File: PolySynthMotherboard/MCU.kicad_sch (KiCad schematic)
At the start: 45 parts, among them J201 SWD Header, J202 USB_C_Receptacle_USB2.0, J203 MIDI_In, J204 MIDI_Thru, J205 MIDI_Out, J401 Micro_SD_Card_Det2, SW201 RST, SW202 BOOT, U201 STM32F411RETx, U202 74HC595, U203 74HC595, U204 4N35, U205 74HC04, Y201 16MHz, Y202 32.768kHZ

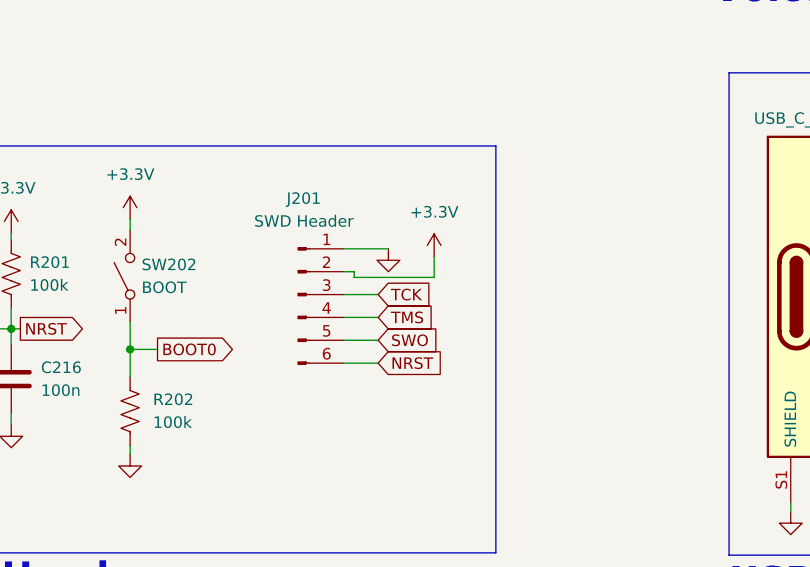
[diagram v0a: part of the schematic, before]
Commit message: board layout
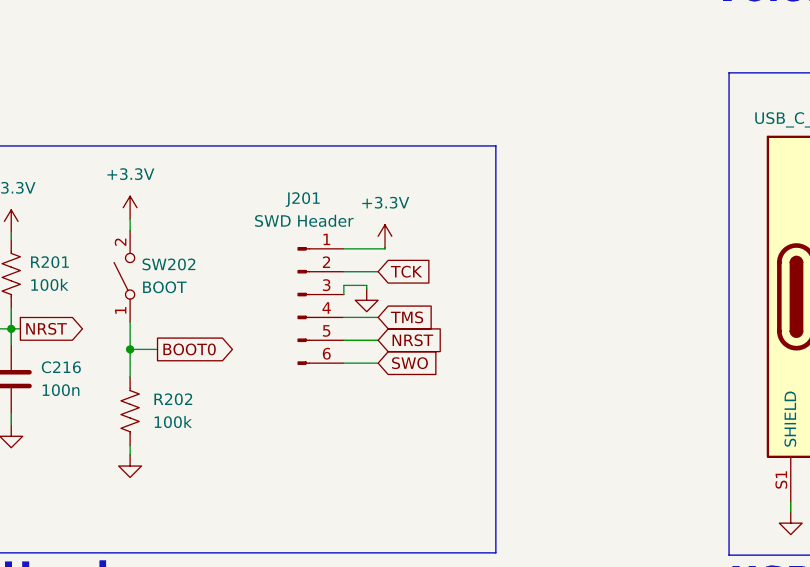
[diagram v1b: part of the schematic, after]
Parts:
- D201: footprint Diode_THT:D_DO-35_SOD27_P7.62mm_Horizontal -> Diode_SMD:D_SOD-123
- U205: footprint PCM_Package_SO_AKL:SOIC-14_3.9x8.7mm_P1.27mm -> Package_SO:SOIC-14_3.9x8.7mm_P1.27mm
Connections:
- net +3.3V: now also J201.1 (Pin_1); no longer J201.2 (Pin_2)
- net GND: now also J201.3 (Pin_3); no longer J201.1 (Pin_1)
- net NRST: now also J201.5 (Pin_5); no longer J201.6 (Pin_6)
- net SWO: now also J201.6 (Pin_6); no longer J201.5 (Pin_5)
- net TCK: now also J201.2 (Pin_2); no longer J201.3 (Pin_3)
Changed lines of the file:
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@@
     (stroke (width 0) (type default))
   )
+  (wire (pts (xy 115.951 196.342) (xy 115.951 196.723))
+    (stroke (width 0) (type default))
+  )
   (wire (pts (xy 121.158 93.218) (xy 123.698 93.218))
     (stroke (width 0) (type default))
@@
     (stroke (width 0) (type default))
   )
-  (wire (pts (xy 114.554 194.818) (xy 114.554 195.453))
-    (stroke (width 0) (type default))
-  )
   (wire (pts (xy 34.29 109.474) (xy 34.29 121.92))
     (stroke (width 0) (type default))
@@
     (stroke (width 0) (type default))
   )
-  (wire (pts (xy 113.411 197.358) (xy 117.221 197.358))
+  (wire (pts (xy 113.411 194.818) (xy 117.221 194.818))
     (stroke (width 0) (type default))
   )
@@
     (stroke (width 0) (type default))
   )
-  (wire (pts (xy 114.554 195.453) (xy 123.444 195.453))
-    (stroke (width 0) (type default))
-  )
   (wire (pts (xy 81.026 85.598) (xy 85.598 85.598))
     (stroke (width 0) (type default))
@@
     (stroke (width 0) (type default))
   )
+  (wire (pts (xy 113.411 196.342) (xy 115.951 196.342))
+    (stroke (width 0) (type default))
+  )
   (wire (pts (xy 121.158 65.278) (xy 156.718 65.278))
     (stroke (width 0) (type default))
@@
     (stroke (width 0) (type default))
   )
-  (wire (pts (xy 113.411 194.818) (xy 114.554 194.818))
-    (stroke (width 0) (type default))
-  )
   (wire (pts (xy 200.914 81.026) (xy 204.724 81.026))
     (stroke (width 0) (type default))
@@
     (stroke (width 0) (type default))
   )
-  (wire (pts (xy 123.444 195.453) (xy 123.444 193.167))
-    (stroke (width 0) (type default))
-  )
   (wire (pts (xy 200.406 134.874) (xy 203.454 134.874))
     (stroke (width 0) (type default))
@@
     (stroke (width 0) (type default))
   )
+  (wire (pts (xy 113.411 197.358) (xy 113.411 196.342))
+    (stroke (width 0) (type default))
+  )
   (wire (pts (xy 83.566 113.538) (xy 85.598 113.538))
     (stroke (width 0) (type default))
@@
     (stroke (width 0) (type default))
   )
-  (wire (pts (xy 113.411 204.978) (xy 117.221 204.978))
+  (wire (pts (xy 113.411 202.438) (xy 117.221 202.438))
     (stroke (width 0) (type default))
   )
@@
     (stroke (width 0) (type default))
   )
+  (wire (pts (xy 113.411 192.278) (xy 117.983 192.278))
+    (stroke (width 0) (type default))
+  )
   (wire (pts (xy 46.482 54.356) (xy 46.482 57.15))
     (stroke (width 0) (type default))
@@
     (stroke (width 0) (type default))
   )
-  (wire (pts (xy 113.411 202.438) (xy 117.221 202.438))
+  (wire (pts (xy 113.411 204.978) (xy 117.221 204.978))
     (stroke (width 0) (type default))
   )
@@
     (stroke (width 0) (type default))
   )
+  (wire (pts (xy 117.983 192.278) (xy 117.983 192.151))
+    (stroke (width 0) (type default))
+  )
   (wire (pts (xy 76.454 201.168) (xy 76.454 202.946))
     (stroke (width 0) (type default))
@@
     (stroke (width 0) (type default))
   )
-  (wire (pts (xy 113.411 192.278) (xy 118.364 192.278))
-    (stroke (width 0) (type default))
-  )
   (wire (pts (xy 279.654 50.419) (xy 286.639 50.419))
     (stroke (width 0) (type default))
@@
     )
   )
-  (global_label "SWO" (shape input) (at 117.221 202.438 0) (fields_autoplaced)
+  (global_label "SWO" (shape input) (at 117.221 204.978 0) (fields_autoplaced)
     (effects (font (size 1.27 1.27)) (justify left))
-    (property "Intersheetrefs" "${INTERSHEET_REFS}" (at 124.1976 202.438 0)
+    (property "Intersheetrefs" "${INTERSHEET_REFS}" (at 124.1976 204.978 0)
       (effects (font (size 1.27 1.27)) (justify left) hide)
     )
@@
     )
   )
-  (global_label "TCK" (shape input) (at 117.221 197.358 0) (fields_autoplaced)
+  (global_label "TCK" (shape input) (at 117.221 194.818 0) (fields_autoplaced)
     (effects (font (size 1.27 1.27)) (justify left))
-    (property "Intersheetrefs" "${INTERSHEET_REFS}" (at 123.7138 197.358 0)
+    (property "Intersheetrefs" "${INTERSHEET_REFS}" (at 123.7138 194.818 0)
       (effects (font (size 1.27 1.27)) (justify left) hide)
     )
@@
     )
   )
-  (global_label "NRST" (shape input) (at 117.221 204.978 0) (fields_autoplaced)
+  (global_label "NRST" (shape input) (at 117.221 202.438 0) (fields_autoplaced)
     (effects (font (size 1.27 1.27)) (justify left))
-    (property "Intersheetrefs" "${INTERSHEET_REFS}" (at 124.9838 204.978 0)
+    (property "Intersheetrefs" "${INTERSHEET_REFS}" (at 124.9838 202.438 0)
       (effects (font (size 1.27 1.27)) (justify left) hide)
     )
@@
       (effects (font (size 1.27 1.27)))
     )
-    (property "Footprint" "PCM_Package_SO_AKL:SOIC-14_3.9x8.7mm_P1.27mm" (at 345.059 149.987 0)
+    (property "Footprint" "Package_SO:SOIC-14_3.9x8.7mm_P1.27mm" (at 345.059 149.987 0)
       (effects (font (size 1.27 1.27)) hide)
     )
@@
       (effects (font (size 1.27 1.27)) (justify right))
     )
-    (property "Footprint" "Diode_THT:D_DO-35_SOD27_P7.62mm_Horizontal" (at 353.695 52.705 0)
+    (property "Footprint" "Diode_SMD:D_SOD-123" (at 353.695 52.705 0)
       (effects (font (size 1.27 1.27)) hide)
     )
@@
       (effects (font (size 1.27 1.27)))
     )
-    (property "Footprint" "PCM_Package_SO_AKL:SOIC-14_3.9x8.7mm_P1.27mm" (at 347.091 84.074 0)
+    (property "Footprint" "Package_SO:SOIC-14_3.9x8.7mm_P1.27mm" (at 347.091 84.074 0)
       (effects (font (size 1.27 1.27)) hide)
     )
@@
       (effects (font (size 1.27 1.27)))
     )
-    (property "Footprint" "PCM_Package_SO_AKL:SOIC-14_3.9x8.7mm_P1.27mm" (at 363.347 84.074 0)
+    (property "Footprint" "Package_SO:SOIC-14_3.9x8.7mm_P1.27mm" (at 363.347 84.074 0)
       (effects (font (size 1.27 1.27)) hide)
     )
@@
       (effects (font (size 1.27 1.27)) (justify left))
     )
-    (property "Footprint" "PCM_Package_SO_AKL:SOIC-14_3.9x8.7mm_P1.27mm" (at 387.731 151.511 0)
+    (property "Footprint" "Package_SO:SOIC-14_3.9x8.7mm_P1.27mm" (at 387.731 151.511 0)
       (effects (font (size 1.27 1.27)) hide)
     )
@@
       (effects (font (size 1.27 1.27)))
     )
-    (property "Footprint" "PCM_Package_SO_AKL:SOIC-14_3.9x8.7mm_P1.27mm" (at 361.696 149.987 0)
+    (property "Footprint" "Package_SO:SOIC-14_3.9x8.7mm_P1.27mm" (at 361.696 149.987 0)
       (effects (font (size 1.27 1.27)) hide)
     )
@@
     )
   )
-  (symbol (lib_id "power:GND") (at 118.364 192.278 0) (unit 1)
+  (symbol (lib_id "power:GND") (at 115.951 196.723 0) (unit 1)
     (in_bom yes) (on_board yes) (dnp no) (fields_autoplaced)
-    (property "Reference" "#PWR0239" (at 118.364 198.628 0)
+    (property "Reference" "#PWR0239" (at 115.951 203.073 0)
       (effects (font (size 1.27 1.27)) hide)
     )
-    (property "Value" "GND" (at 118.364 196.088 0)
+    (property "Value" "GND" (at 115.951 200.533 0)
       (effects (font (size 1.27 1.27)) hide)
     )
-    (property "Footprint" "" (at 118.364 192.278 0)
+    (property "Footprint" "" (at 115.951 196.723 0)
       (effects (font (size 1.27 1.27)) hide)
     )
-    (property "Datasheet" "" (at 118.364 192.278 0)
+    (property "Datasheet" "" (at 115.951 196.723 0)
       (effects (font (size 1.27 1.27)) hide)
     )
@@
     )
   )
-  (symbol (lib_id "power:+3.3V") (at 123.444 193.167 0) (unit 1)
+  (symbol (lib_id "power:+3.3V") (at 117.983 192.151 0) (unit 1)
     (in_bom yes) (on_board yes) (dnp no) (fields_autoplaced)
-    (property "Reference" "#PWR0240" (at 123.444 196.977 0)
+    (property "Reference" "#PWR0240" (at 117.983 195.961 0)
       (effects (font (size 1.27 1.27)) hide)
     )
-    (property "Value" "+3.3V" (at 123.444 188.214 0)
+    (property "Value" "+3.3V" (at 117.983 187.198 0)
       (effects (font (size 1.27 1.27)))
     )
-    (property "Footprint" "" (at 123.444 193.167 0)
+    (property "Footprint" "" (at 117.983 192.151 0)
       (effects (font (size 1.27 1.27)) hide)
     )
-    (property "Datasheet" "" (at 123.444 193.167 0)
+    (property "Datasheet" "" (at 117.983 192.151 0)
       (effects (font (size 1.27 1.27)) hide)
     )
@@
       (effects (font (size 1.27 1.27)))
     )
-    (property "Footprint" "PCM_Package_SO_AKL:SOIC-14_3.9x8.7mm_P1.27mm" (at 364.871 113.792 0)
+    (property "Footprint" "Package_SO:SOIC-14_3.9x8.7mm_P1.27mm" (at 364.871 113.792 0)
       (effects (font (size 1.27 1.27)) hide)
     )
@@
       (effects (font (size 1.27 1.27)))
     )
-    (property "Footprint" "PCM_Package_SO_AKL:SOIC-14_3.9x8.7mm_P1.27mm" (at 346.71 113.792 0)
+    (property "Footprint" "Package_SO:SOIC-14_3.9x8.7mm_P1.27mm" (at 346.71 113.792 0)
       (effects (font (size 1.27 1.27)) hide)
     )

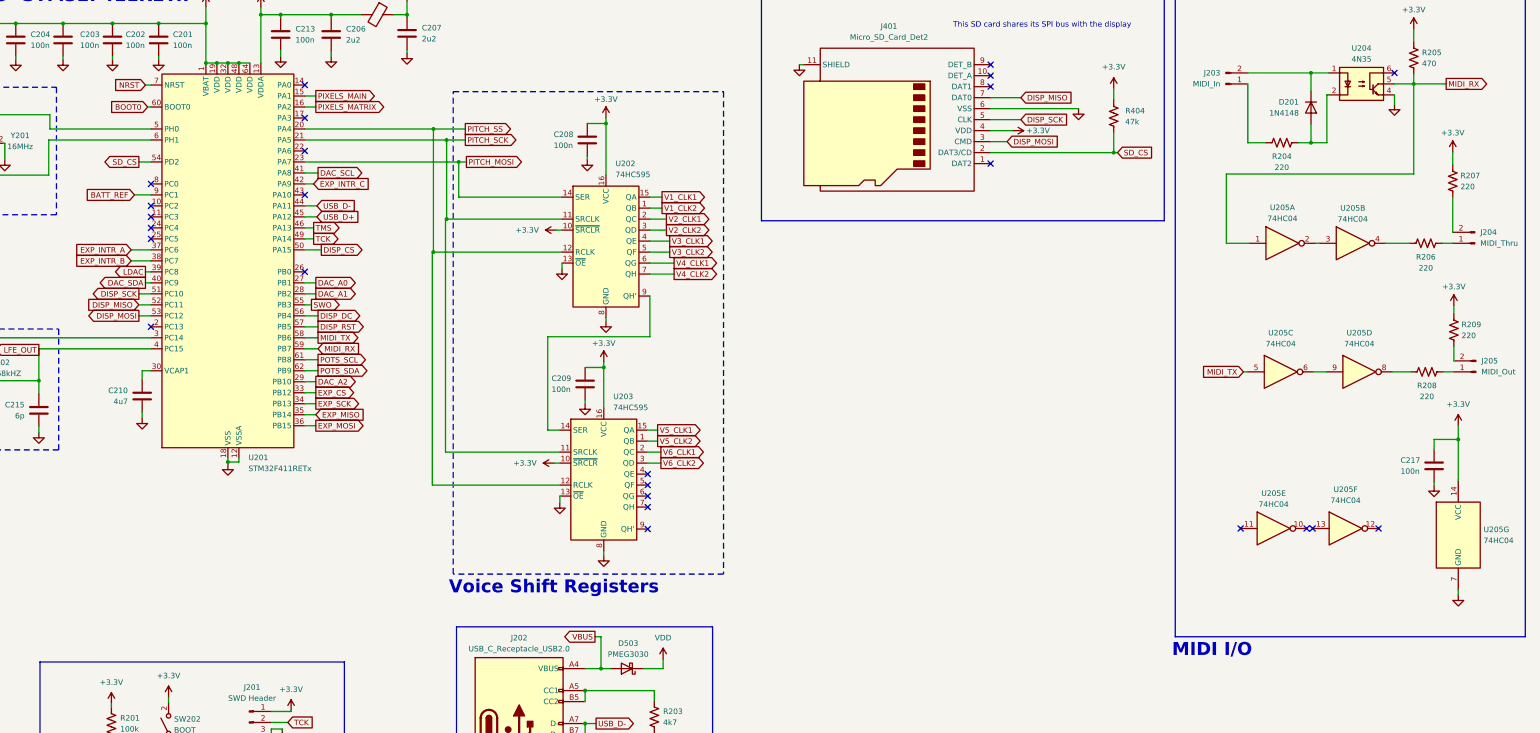
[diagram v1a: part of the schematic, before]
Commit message: new voice board proj
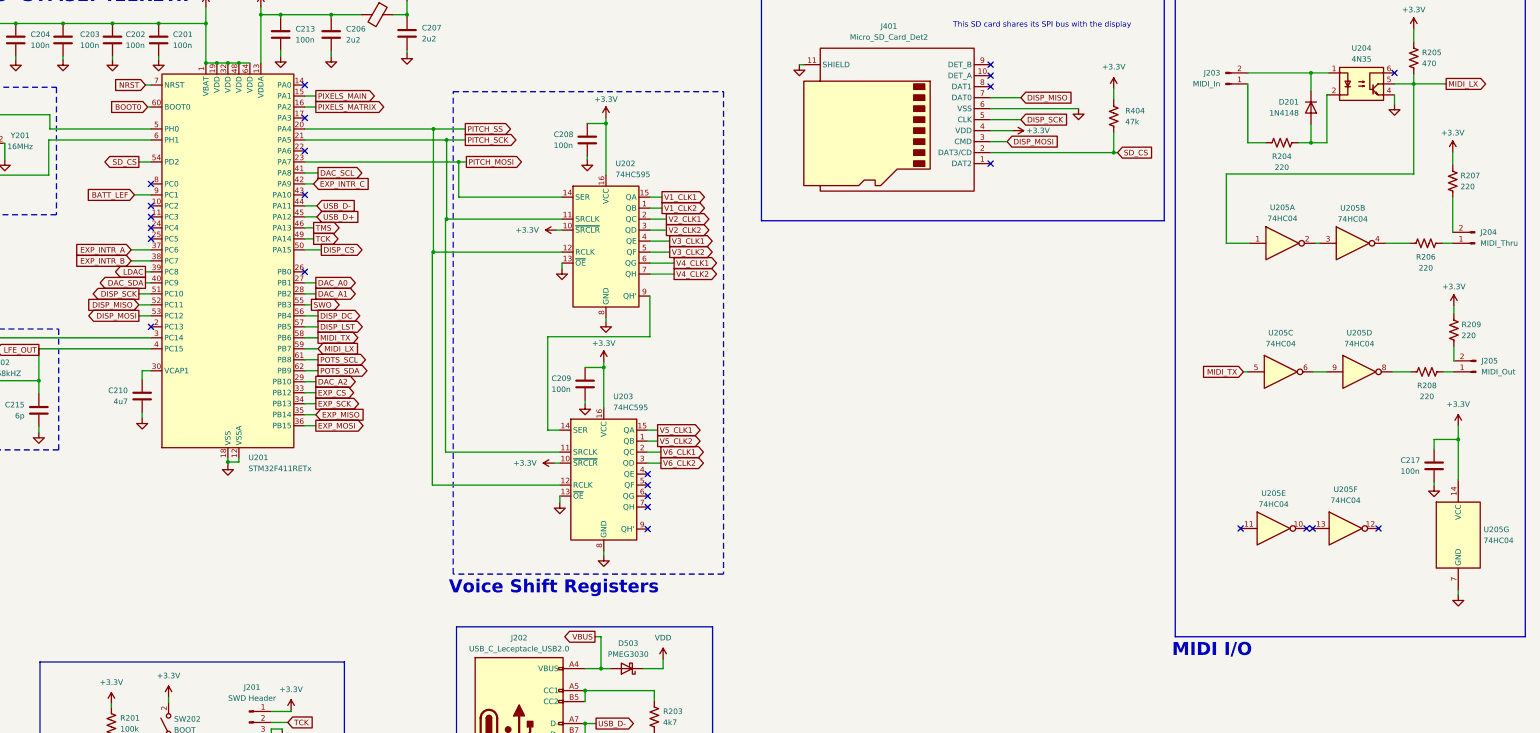
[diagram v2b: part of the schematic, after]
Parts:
- J202: value USB_C_Receptacle_USB2.0 -> USB_C_Leceptacle_USB2.0
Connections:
- net BATT_REF renamed BATT_LEF
- net DISP_RST renamed DISP_LST
- net MIDI_RX renamed MIDI_LX
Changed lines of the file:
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@@
     )
   )
-  (global_label "MIDI_RX" (shape input) (at 124.206 108.458 0) (fields_autoplaced)
+  (global_label "MIDI_LX" (shape input) (at 124.206 108.458 0) (fields_autoplaced)
     (effects (font (size 1.27 1.27)) (justify left))
     (property "Intersheetrefs" "${INTERSHEET_REFS}" (at 134.5693 108.458 0)
@@
     )
   )
-  (global_label "MIDI_RX" (shape output) (at 384.937 47.244 0) (fields_autoplaced)
+  (global_label "MIDI_LX" (shape output) (at 384.937 47.244 0) (fields_autoplaced)
     (effects (font (size 1.27 1.27)) (justify left))
     (property "Intersheetrefs" "${INTERSHEET_REFS}" (at 395.3003 47.244 0)
@@
     )
   )
-  (global_label "BATT_REF" (shape input) (at 81.788 72.898 180) (fields_autoplaced)
+  (global_label "BATT_LEF" (shape input) (at 81.788 72.898 180) (fields_autoplaced)
     (effects (font (size 1.27 1.27)) (justify right))
     (property "Intersheetrefs" "${INTERSHEET_REFS}" (at 70.0338 72.898 0)
@@
     )
   )
-  (global_label "DISP_RST" (shape output) (at 124.206 103.378 0) (fields_autoplaced)
+  (global_label "DISP_LST" (shape output) (at 124.206 103.378 0) (fields_autoplaced)
     (effects (font (size 1.27 1.27)) (justify left))
     (property "Intersheetrefs" "${INTERSHEET_REFS}" (at 135.9602 103.378 0)
@@
       (effects (font (size 1.27 1.27)))
     )
-    (property "Value" "USB_C_Receptacle_USB2.0" (at 170.688 177.8 0)
-      (effects (font (size 1.27 1.27)))
-    )
+    (property "Value" "USB_C_Leceptacle_USB2.0" (at 170.688 177.8 0)
+      (effects (font (size 1.27 1.27)))
+    )
